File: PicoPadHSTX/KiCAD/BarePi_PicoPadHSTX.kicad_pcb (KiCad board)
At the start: 2 copper layers, 65 x 48 mm, 17 parts, among them IC1 Raspberry Pi Pico 2, J1 OUT, J2 DISPLAY

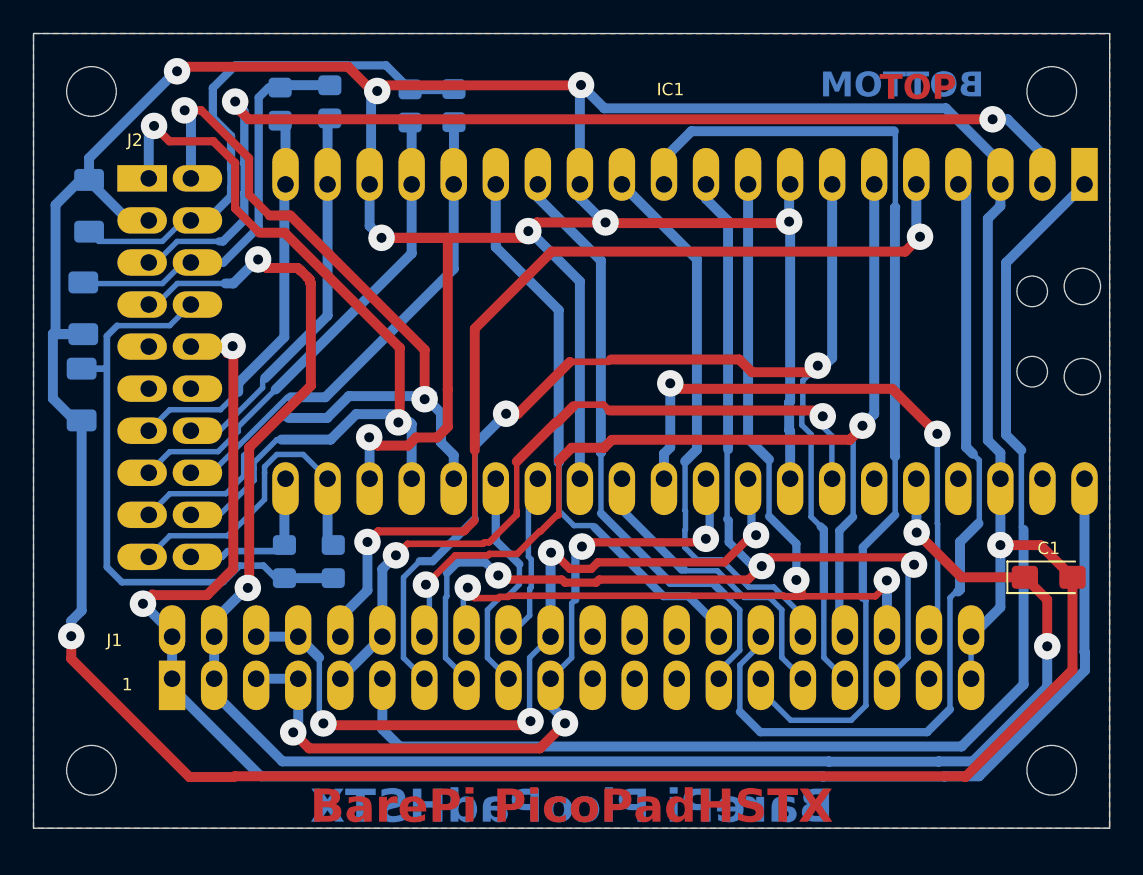
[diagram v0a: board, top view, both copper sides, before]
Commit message: init
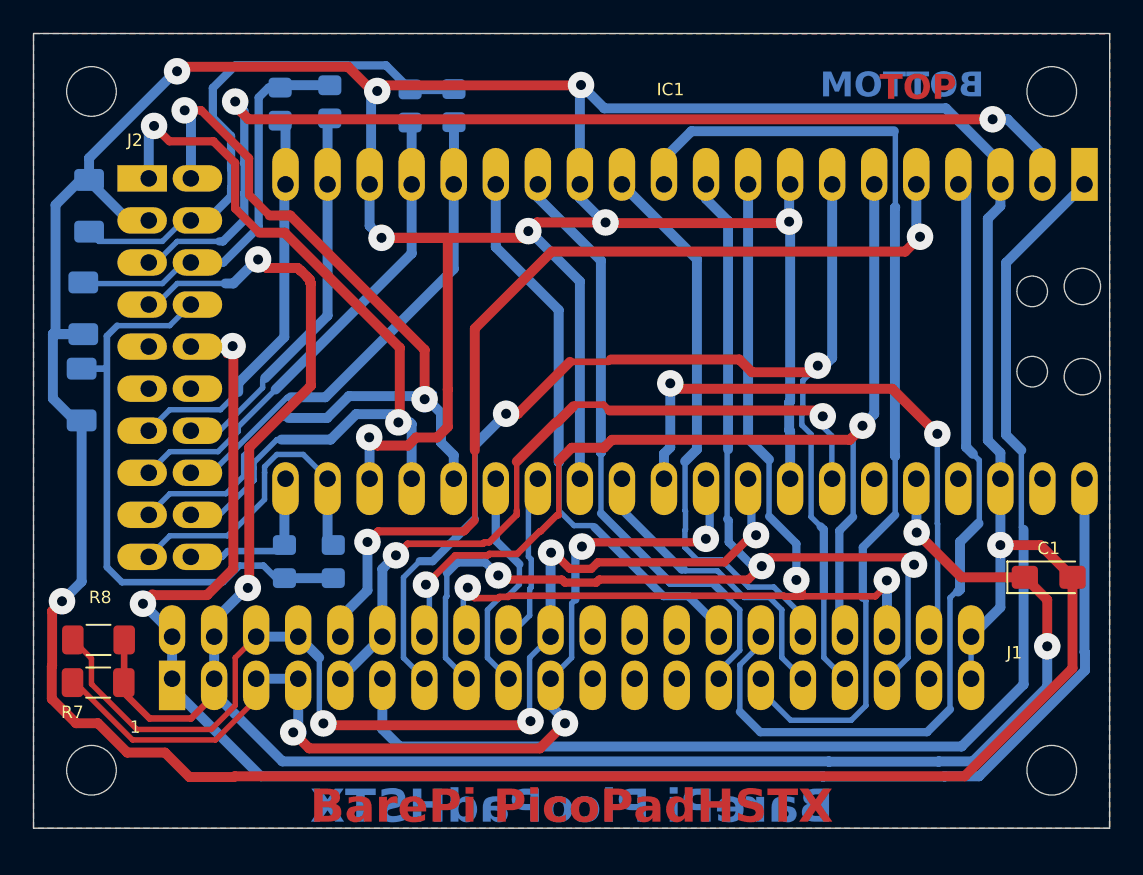
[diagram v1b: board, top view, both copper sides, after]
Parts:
- added R7: 15K, Resistor_SMD:R_1206_3216Metric_Pad1.30x1.75mm_HandSolder, F.Cu at (3.90, 39.2)
- added R8: 15K, Resistor_SMD:R_1206_3216Metric_Pad1.30x1.75mm_HandSolder, F.Cu at (3.92, 36.6)
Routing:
- net /SCL/RX: track 49.2 -> 67.4 mm
- net /SDA/TX: track 47.0 -> 61.8 mm
- net /3V3: track 110.9 -> 121.4 mm
- net /GND: track 311.5 -> 314.5 mm
